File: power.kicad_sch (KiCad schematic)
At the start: 44 parts, among them J2 UJ20-C-H-G-SMT-1-P16-TR, U2 MCP73871, U3 AP2112K-3.3, U4 MAX17048G_T10, U5 USBLC6-2SC6, U9 USBLC6-2SC6

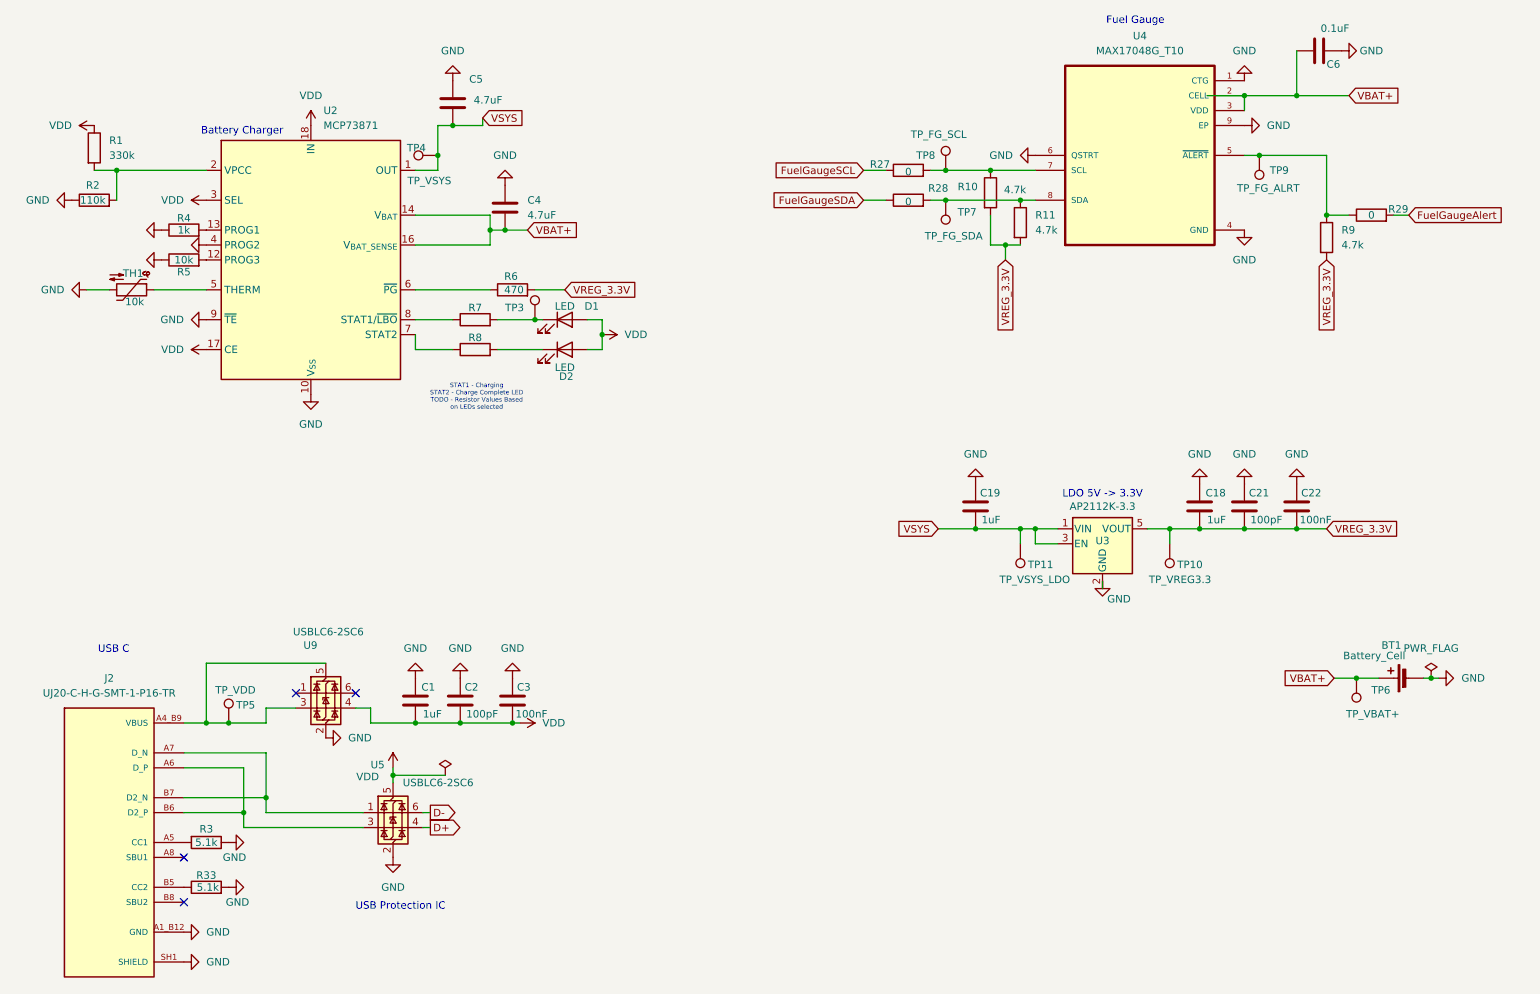
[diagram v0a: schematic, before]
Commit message: Update speaker PCB design
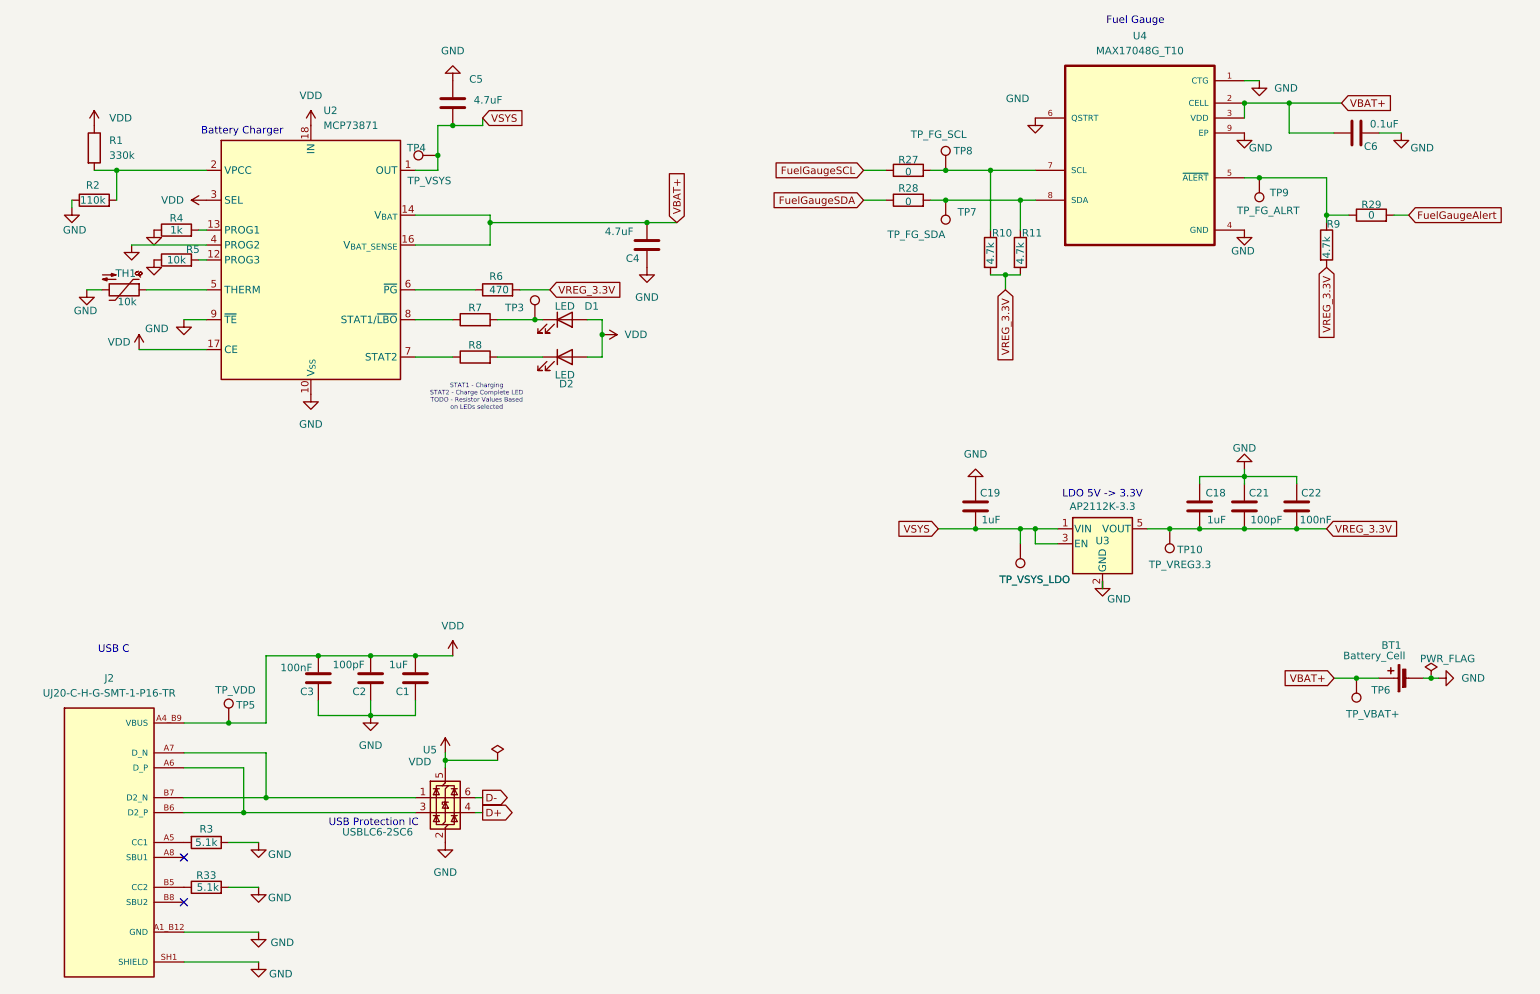
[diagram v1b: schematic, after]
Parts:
- removed U9: USBLC6-2SC6, Package_TO_SOT_SMD:SOT-23-6, symbol Power_Protection:USBLC6-2SC6
- renumbered TP11 to TP_VSYS_LDO
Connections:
- net VDD: now also J2.A4_B9 (VBUS), J2.B4_A9 (VBUS), TP5.1
- no-connect marks 4 -> 2
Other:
- moved on the sheet: C1, C2, C3, C4, C6, D2, R10, R11, R4, R5, R6, R8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
